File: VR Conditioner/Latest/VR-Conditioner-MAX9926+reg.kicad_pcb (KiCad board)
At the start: 2 copper layers, 19.7 x 19.7 mm, 22 parts, among them J1 8-pin header, J2 Edge, U1 MAX9926UAEE+, U2 AMS1117CD-5.0

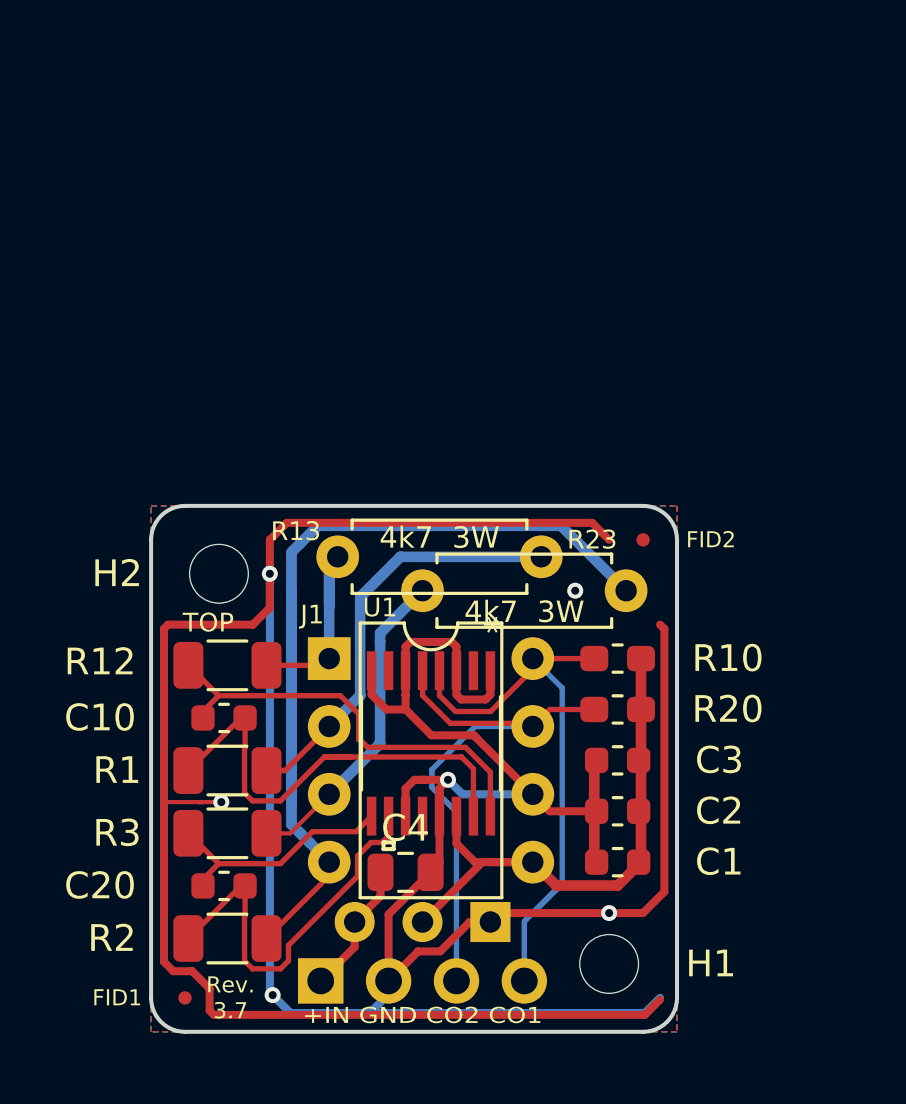
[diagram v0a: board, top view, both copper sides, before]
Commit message: Update original vr conditioner
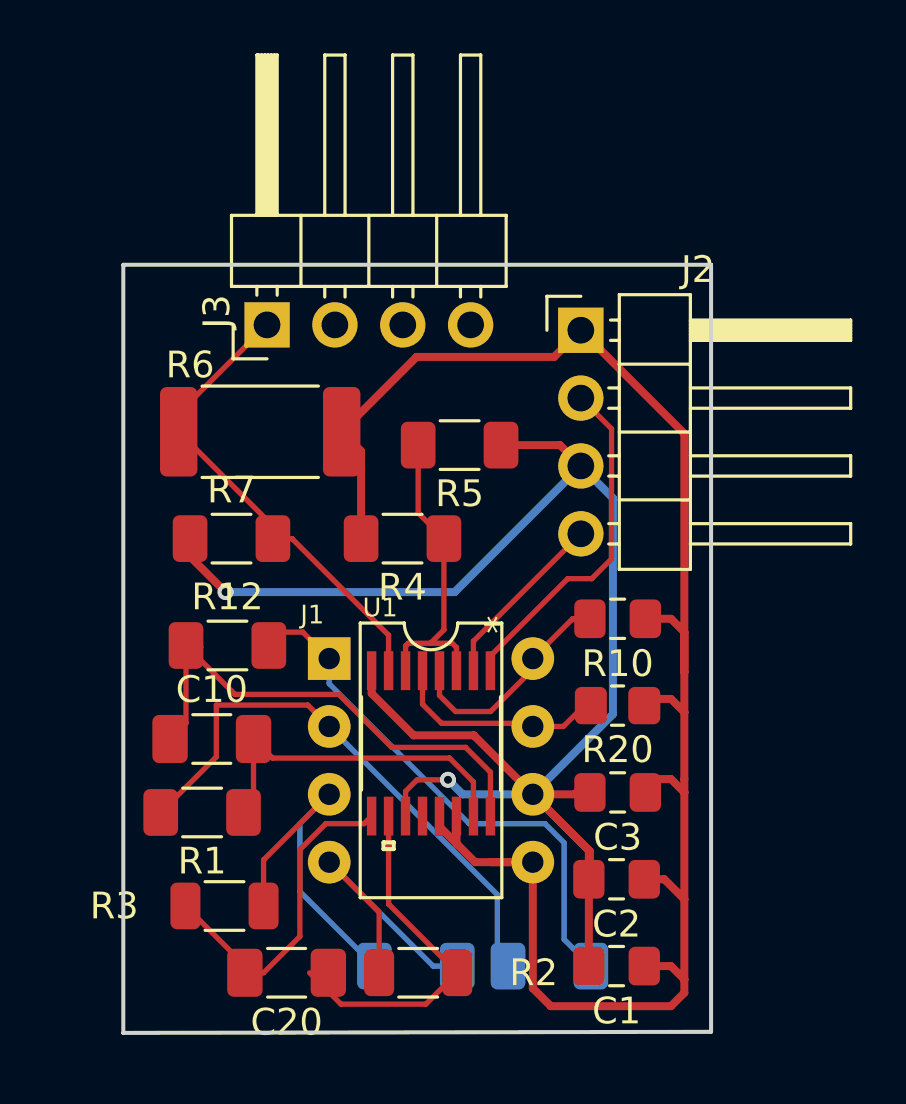
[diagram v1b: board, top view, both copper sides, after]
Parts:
- removed C4: 10u, Capacitor_SMD:C_0805_2012Metric
- removed FID1, FID2: Fiducial, Fiducial:Fiducial_0.5mm_Mask1mm
- removed H1, H2: MountingHole, MountingHole:MountingHole_2.2mm_M2
- removed U2: AMS1117CD-5.0, Package_TO_SOT_THT:TO-92_Inline_Wide
- added J3: Edge, Connector_PinHeader_2.54mm:PinHeader_1x04_P2.54mm_Horizontal, F.Cu at (116.7, 89.7)
- added R4: 10k, Resistor_SMD:R_1206_3216Metric_Pad1.30x1.75mm_HandSolder, F.Cu at (121.8, 97.7)
- added R5: 10k, Resistor_SMD:R_1206_3216Metric_Pad1.30x1.75mm_HandSolder, F.Cu at (123.9, 94.2)
- added R6: 1k, Resistor_SMD:R_2512_6332Metric_Pad1.40x3.35mm_HandSolder, F.Cu at (116.5, 93.7)
- added R7: 10k, Resistor_SMD:R_1206_3216Metric_Pad1.30x1.75mm_HandSolder, F.Cu at (115.4, 97.7)
- C1, C2, C3: footprint Capacitor_SMD:C_0603_1608Metric -> Capacitor_SMD:C_0805_2012Metric_Pad1.18x1.45mm_HandSolder
- C10, C20: footprint Capacitor_SMD:C_0603_1608Metric -> Capacitor_SMD:C_1206_3216Metric_Pad1.33x1.80mm_HandSolder
- J2: moved to F.Cu
- R1, R12: footprint Resistor_SMD:R_1206_3216Metric -> Resistor_SMD:R_1206_3216Metric_Pad1.30x1.75mm_HandSolder
- R10: value 1k -> 560; footprint Resistor_SMD:R_0603_1608Metric_Pad1.05x0.95mm_HandSolder -> Capacitor_SMD:C_0805_2012Metric_Pad1.18x1.45mm_HandSolder
- R13, R23: footprint Resistor_THT:R_Axial_DIN0207_L6.3mm_D2.5mm_P7.62mm_Horizontal -> Resistor_SMD:R_1206_3216Metric_Pad1.30x1.75mm_HandSolder; moved to B.Cu
- R20: value 1k -> 560; footprint Resistor_SMD:R_0603_1608Metric_Pad1.05x0.95mm_HandSolder -> Resistor_SMD:R_0805_2012Metric_Pad1.20x1.40mm_HandSolder
- moved J2 26.2 mm to (128.5, 89.9), turned to 0 degrees
- moved R13 17.2 mm to (127.3, 113.7), turned to 180 degrees
- moved R23 14.1 mm to (122.3, 113.7)
- moved R2 7.25 mm to (122.4, 114.0), turned to 180 degrees
- moved C20 4.01 mm to (117.5, 114.0)
- moved C1 3.89 mm to (129.8, 113.7)
- moved R3 2.72 mm to (115.1, 111.5)
- moved C2 2.55 mm to (129.8, 110.5)
- moved R1 1.83 mm to (114.3, 108.0), turned to 180 degrees
- moved R10 1.49 mm to (129.9, 100.7)
- moved C3 1.20 mm to (129.9, 107.2)
- moved C10 0.91 mm to (114.7, 105.2)
- moved R12 0.74 mm to (115.3, 101.7)
- moved R20 0.15 mm to (129.9, 104.0)
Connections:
- J2 pad 1: +12V -> VCC
- J2 pad 2: GND -> Net-(J2-Pin_2)
- J2 pad 3: /COUT2 -> GND
- J2 pad 4: /COUT1 -> Net-(J2-Pin_4)
- U1 pad 1: GND -> Net-(J2-Pin_2)
- U1 pad 12: Net-(U1-Pad12) -> unconnected-(U1-DIRN-Pad12)
- U1 pad 13: GND -> VCC
- U1 pad 2: Net-(U1-Pad2) -> Net-(J2-Pin_4)
- U1 pad 3: GND -> Net-(U1-BIAS1)
- U1 pad 6: GND -> Net-(U1-BIAS1)
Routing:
- net GND: track 148.7 -> 63.5 mm, vias 6 -> 2
- net VCC: track 22.5 -> 71.3 mm
- net Net-(J1-Pin_4): track 38.5 -> 11.6 mm
- net Net-(J3-Pin_1): track 0.00 -> 19.0 mm
- net /COUT1: track 22.7 -> 8.48 mm
- net Net-(J2-Pin_2): track 0.00 -> 13.1 mm
- net Net-(J1-Pin_1): track 7.60 -> 20.3 mm
- net /COUT2: track 20.8 -> 8.33 mm
- net Net-(U1-BIAS1): track 0.00 -> 11.8 mm
- net Net-(J2-Pin_4): track 0.00 -> 6.79 mm
- net Net-(J1-Pin_2): track 15.8 -> 21.2 mm
- net +12V: track 4.99 -> 0.00 mm
- net Net-(U1-IN1-): track 18.1 -> 13.4 mm
- net Net-(U1-IN2+): track 9.65 -> 12.3 mm
- net Net-(U1-IN1+): track 17.0 -> 19.5 mm
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- removed copper zone on B.Cu, net GND
- removed copper zone on F.Cu, net GND
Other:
- board size 19.7 x 19.7 mm -> 22 x 28.8 mm
- net class Default removed
- net class Minimum removed
- net class power removed
- board text removed: "(c)2021 Phill Rogers"
- board text removed: "+IN GND CO2 CO1"
- board text removed: "4k7 3W"
- board text removed: "6-15V+"
- board text removed: "AMS1117CD-5.0"
- board text removed: "Dual VR conditioner"
- board text removed: "Rev. 3.7"
- board text removed: "Speeduino / compatible"
- board text removed: "TOP"
- board text removed: "mode A2"
